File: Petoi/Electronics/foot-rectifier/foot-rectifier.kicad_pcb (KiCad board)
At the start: 2 copper layers, 26 x 20 mm, 6 parts, among them J1 Conn_01x04_Male, J2 Conn_01x02_Male

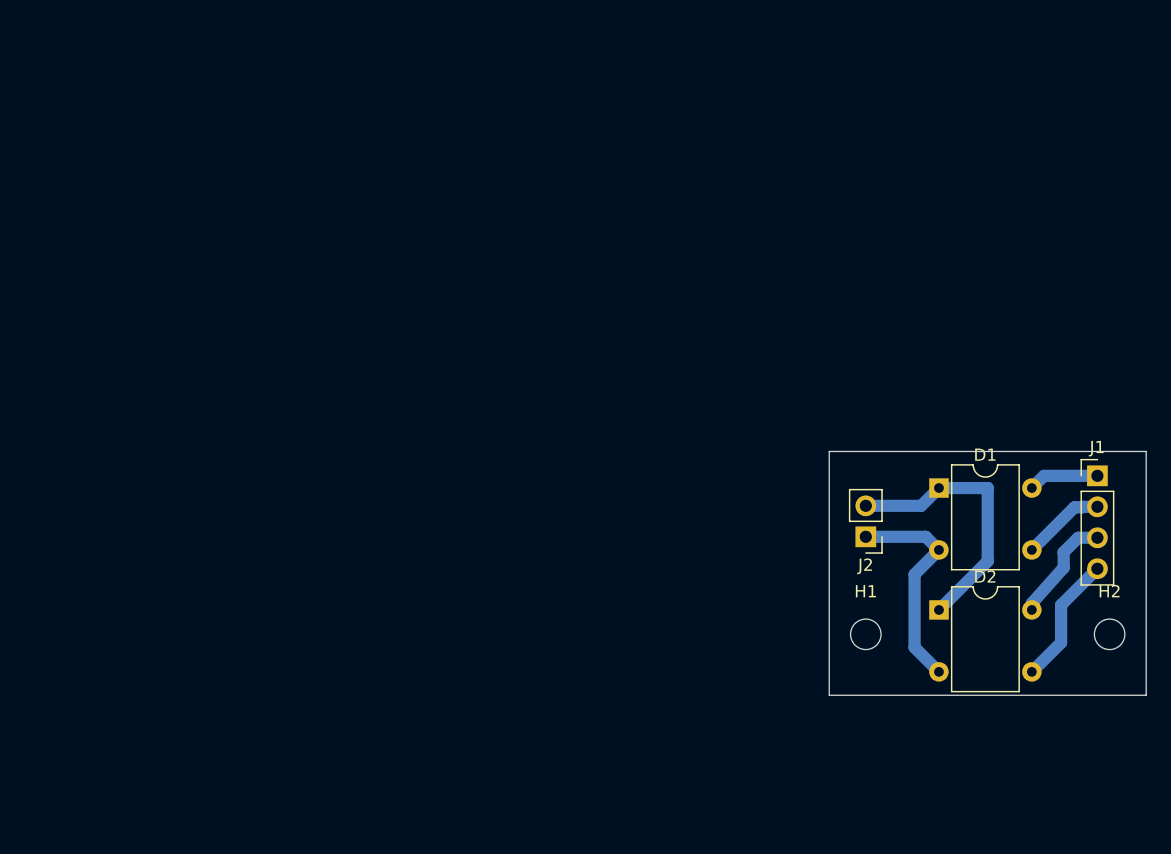
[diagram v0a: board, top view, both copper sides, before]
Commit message: Sally's updated designs.
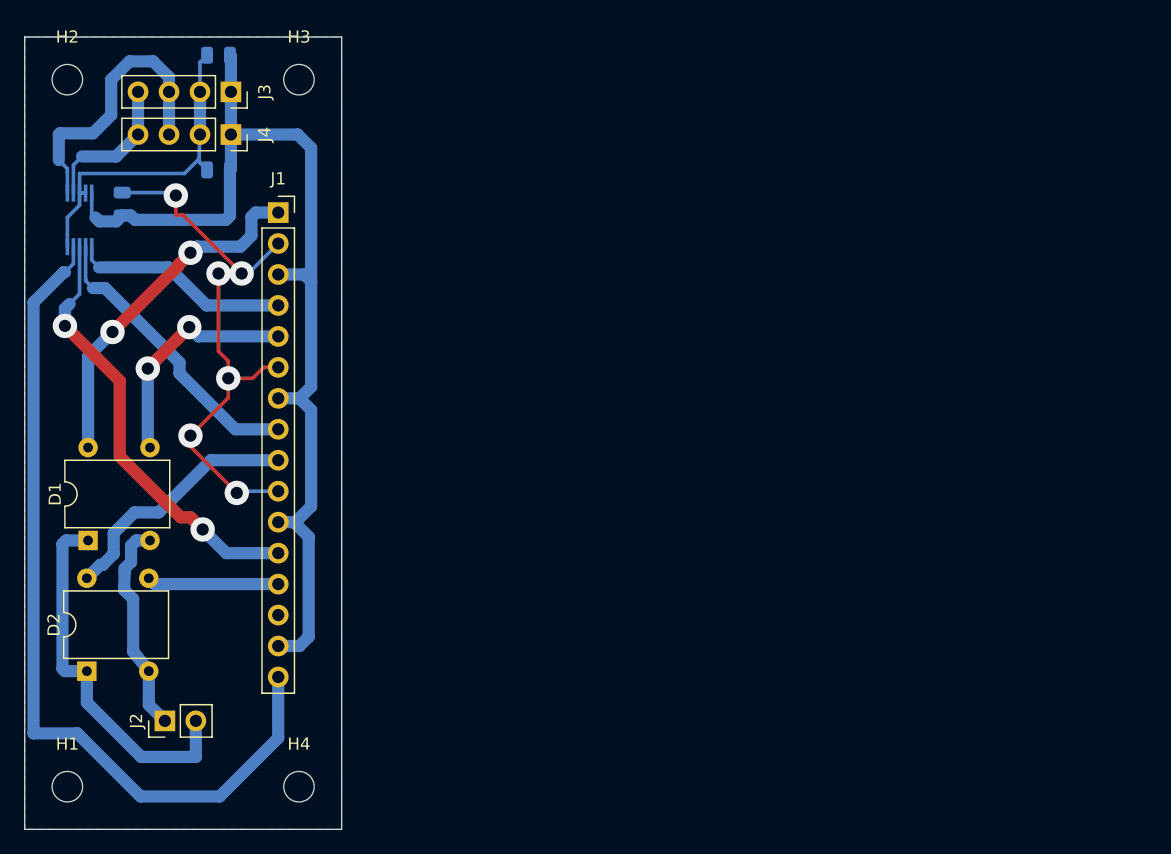
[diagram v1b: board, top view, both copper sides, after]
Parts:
- added C1: 0.1u, Capacitor_SMD:C_0805_2012Metric, B.Cu at (95.9, -54.1)
- added C2: 0.1u, Capacitor_SMD:C_0805_2012Metric, B.Cu at (88.0, -51.3)
- added C3: 0.1u, Capacitor_SMD:C_0805_2012Metric, B.Cu at (95.9, -63.5)
- added H3: MountingHole, MountingHole:MountingHole_2.5mm, F.Cu at (102.5, -61.5)
- added H4: MountingHole, MountingHole:MountingHole_2.5mm, F.Cu at (102.5, -3.50)
- added J3: I2C, Connector_PinSocket_2.54mm:PinSocket_1x04_P2.54mm_Vertical, F.Cu at (96.9, -60.5)
- added J4: range, Connector_PinSocket_2.54mm:PinSocket_1x04_P2.54mm_Vertical, F.Cu at (96.9, -57.0)
- added U1: LTC2990, Package_SO:MSOP-10_3x3mm_P0.5mm, B.Cu at (84.5, -50.0)
- J1: value Conn_01x04_Male -> Legs; footprint Connector_PinHeader_2.54mm:PinHeader_1x04_P2.54mm_Vertical -> Connector_PinSocket_2.54mm:PinSocket_1x16_P2.54mm_Vertical
- J2: value Conn_01x02_Male -> USB pwr out
- moved H2 96.9 mm to (83.5, -61.5)
- moved J1 70.6 mm to (100.8, -50.6)
- moved D2 70.1 mm to (85.1, -13.0), turned to 90 degrees
- moved D1 69.9 mm to (85.2, -23.7), turned to 90 degrees
- moved H1 66.7 mm to (83.5, -3.50)
- moved J2 59.4 mm to (91.5, -8.90), turned to 90 degrees
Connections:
- J1 pad 2: Net-(D1-Pad3) -> GND
- J1 pad 3: Net-(D2-Pad4) -> +3V3
- J1 pad 4: Net-(D2-Pad3) -> Net-(J1-Pad4)
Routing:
- net +3V3: track 0.00 -> 84.8 mm
- net GND: track 0.00 -> 75.6 mm, vias 0 -> 6
- net Net-(J1-Pad16): track 0.00 -> 70.5 mm
- net Net-(J1-Pad12): track 0.00 -> 35.8 mm, vias 0 -> 2
- net Net-(J1-Pad8): track 0.00 -> 24.2 mm
- net SDA: track 0.00 -> 23.6 mm
- net Net-(D1-Pad4): track 5.79 -> 28.9 mm, vias 0 -> 2
- net Net-(J1-Pad4): track 0.00 -> 17.9 mm
- net SCL: track 0.00 -> 12.1 mm
- net Net-(D1-Pad3): track 6.85 -> 19.0 mm, vias 0 -> 2
- net Net-(D2-Pad4): track 8.99 -> 20.7 mm
- net Net-(D1-Pad1): track 22.3 -> 30.9 mm
- added copper zone on B.Cu, net GND
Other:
- board size 26 x 20 mm -> 26 x 65 mm
